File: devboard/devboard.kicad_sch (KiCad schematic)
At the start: 33 parts, among them J1 USB_C_Receptacle_USB2.0_14P, J2 Conn_01x20, J3 Conn_01x20, J4 Conn_01x03, SW1 SW_Push, U1 RP2040, U2 NCP1117-3.3_SOT223, U3 W25Q128JVS, Y1 ASCO

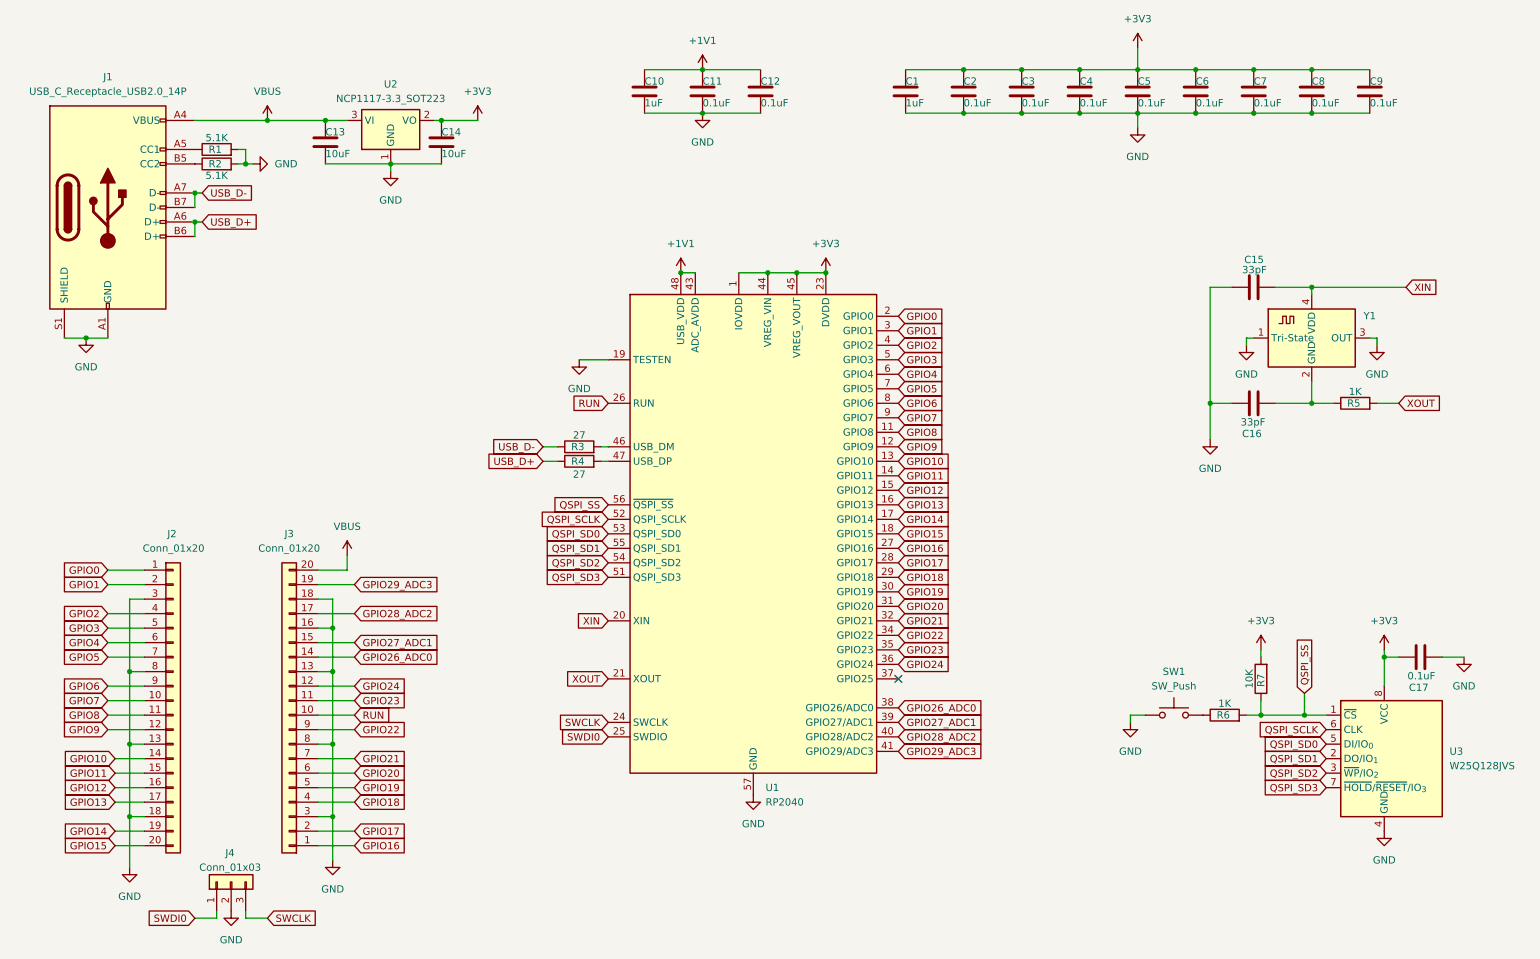
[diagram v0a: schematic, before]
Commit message: PCB routing and changes
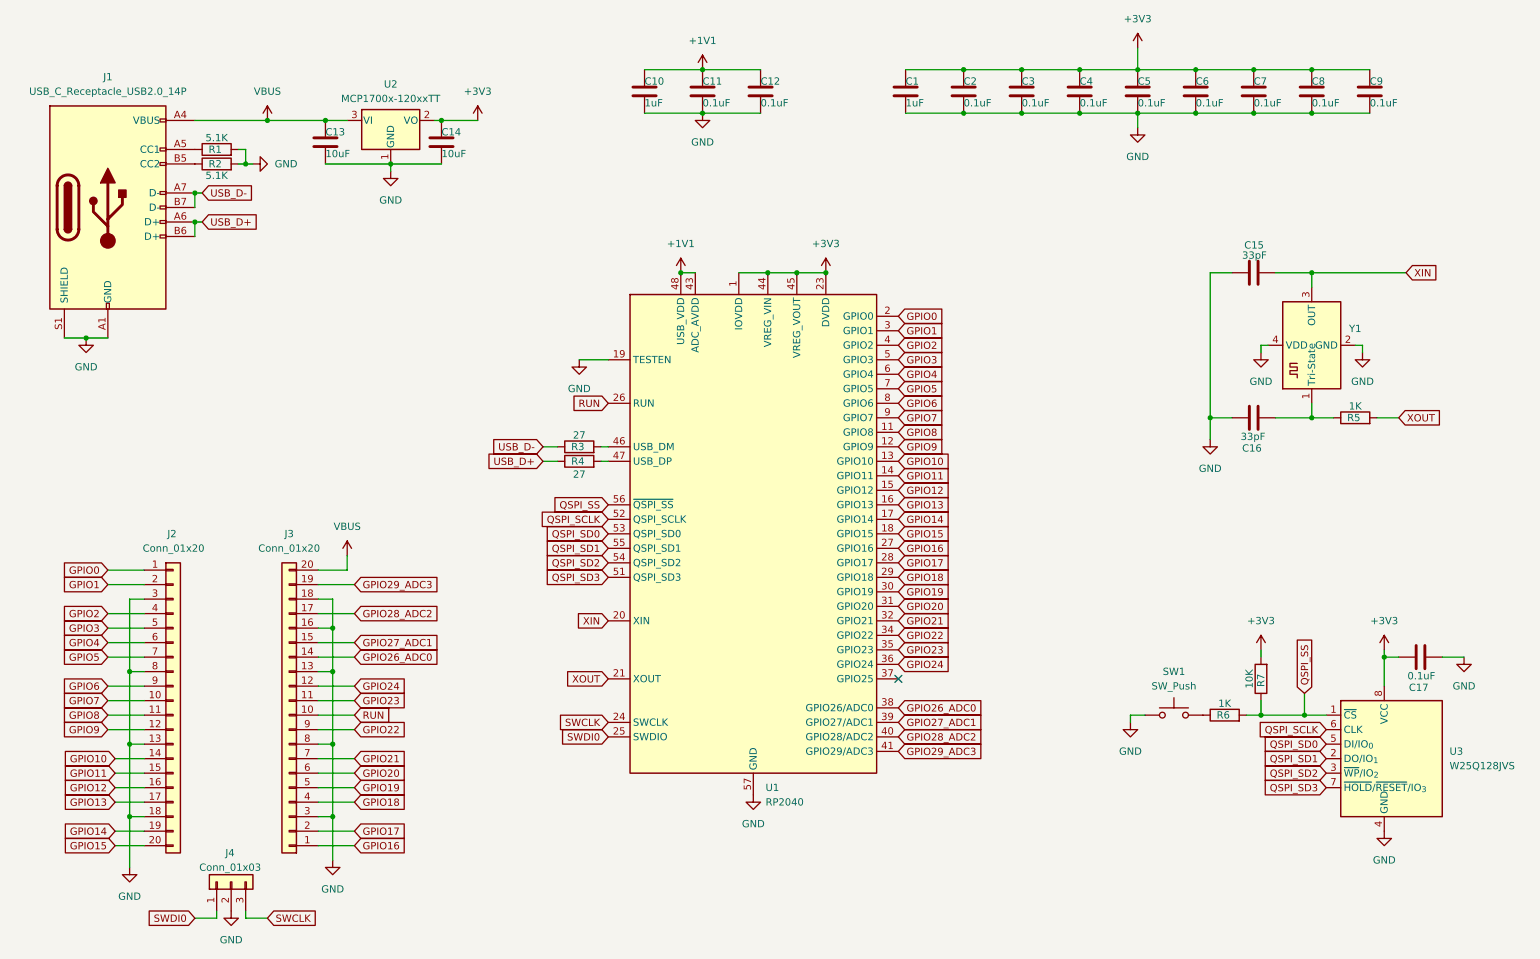
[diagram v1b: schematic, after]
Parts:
- removed U2: NCP1117-3.3_SOT223, Package_TO_SOT_SMD:SOT-223-3_TabPin2, symbol Regulator_Linear:NCP1117-3.3_SOT223
- added U2: MCP1700x-120xxTT, Package_TO_SOT_SMD:SOT-23, symbol Regulator_Linear:MCP1700x-120xxTT
- U3: footprint Package_SO:SOIC-8_5.3x5.3mm_P1.27mm -> Package_SON:Winbond_USON-8-1EP_3x2mm_P0.5mm_EP0.2x1.6mm
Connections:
- net +3V3: now also U2.2 (VO)
- net GND: now also Y1.2 (GND), Y1.4 (VDD), U2.1 (GND); no longer Y1.1 (Tri-State), Y1.3 (OUT)
- net VBUS: now also U2.3 (VI)
- net XIN: now also Y1.3 (OUT); no longer Y1.4 (VDD)
- net at C16.1, R5.1: now also Y1.1 (Tri-State); no longer Y1.2 (GND)
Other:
- moved on the sheet: C15, C16, R5, Y1
